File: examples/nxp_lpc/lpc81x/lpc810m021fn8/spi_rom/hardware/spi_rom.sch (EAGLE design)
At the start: 12 parts, among them IC1 LPC810M021FN8, IC2 25LC640A/P, J1 POWER_JACKPTH_BREAD

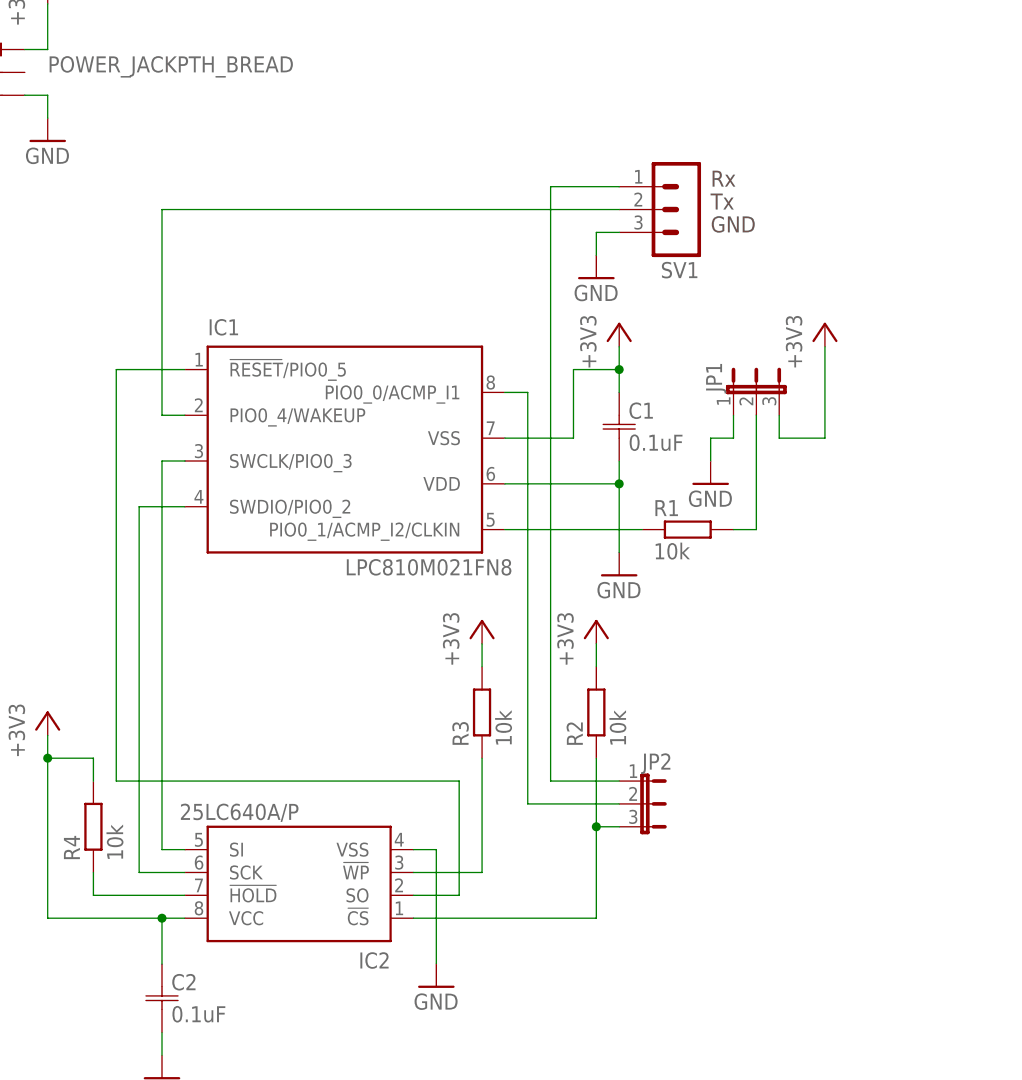
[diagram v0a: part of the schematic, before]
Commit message: Fix schematic.
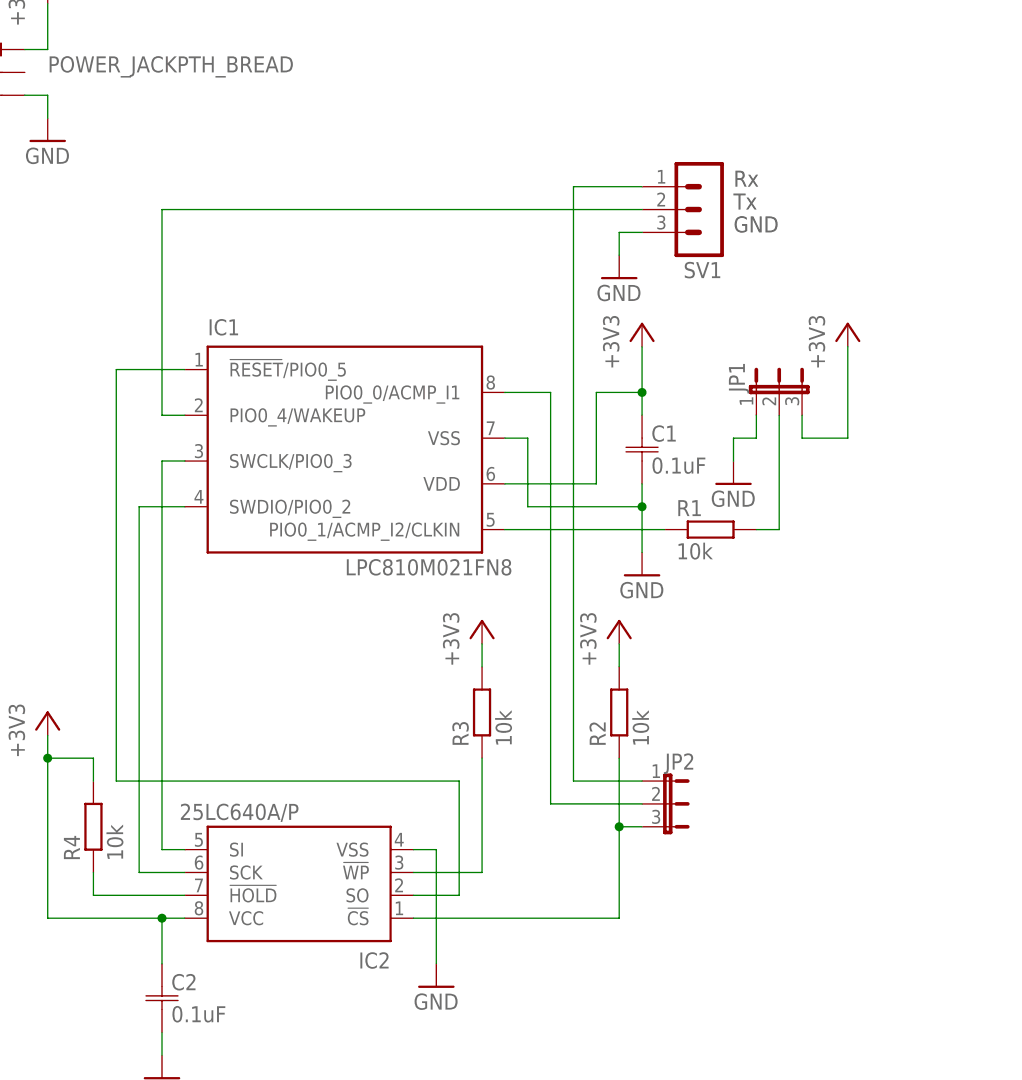
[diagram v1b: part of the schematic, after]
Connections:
- net +3V3: now also IC1.VDD; no longer IC1.VSS
- net GND: now also IC1.VSS; no longer IC1.VDD
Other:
- moved on the sheet: C1, JP1, JP2, R1, R2, SV1
